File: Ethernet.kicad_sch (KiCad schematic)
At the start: 23 parts, among them T1 WE-RJ45_7499010211A, U4 DP83825IRMQR, Y3 ECS-250-12-33-AGN-TR

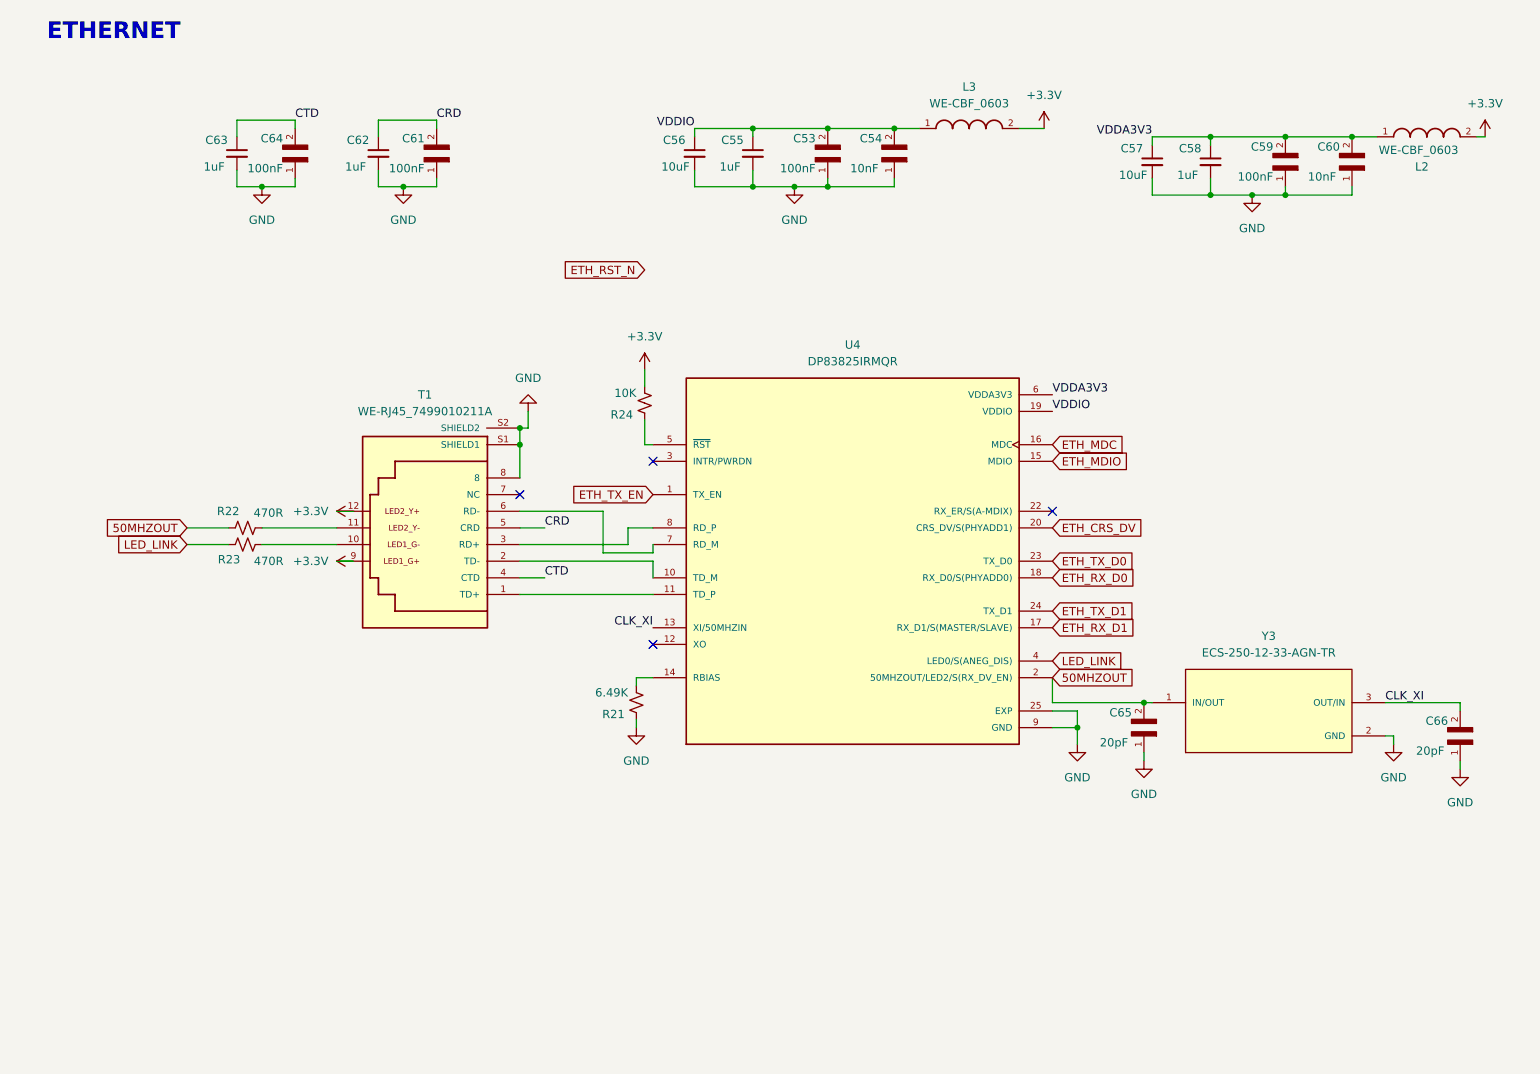
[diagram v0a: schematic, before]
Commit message: schamtic Update
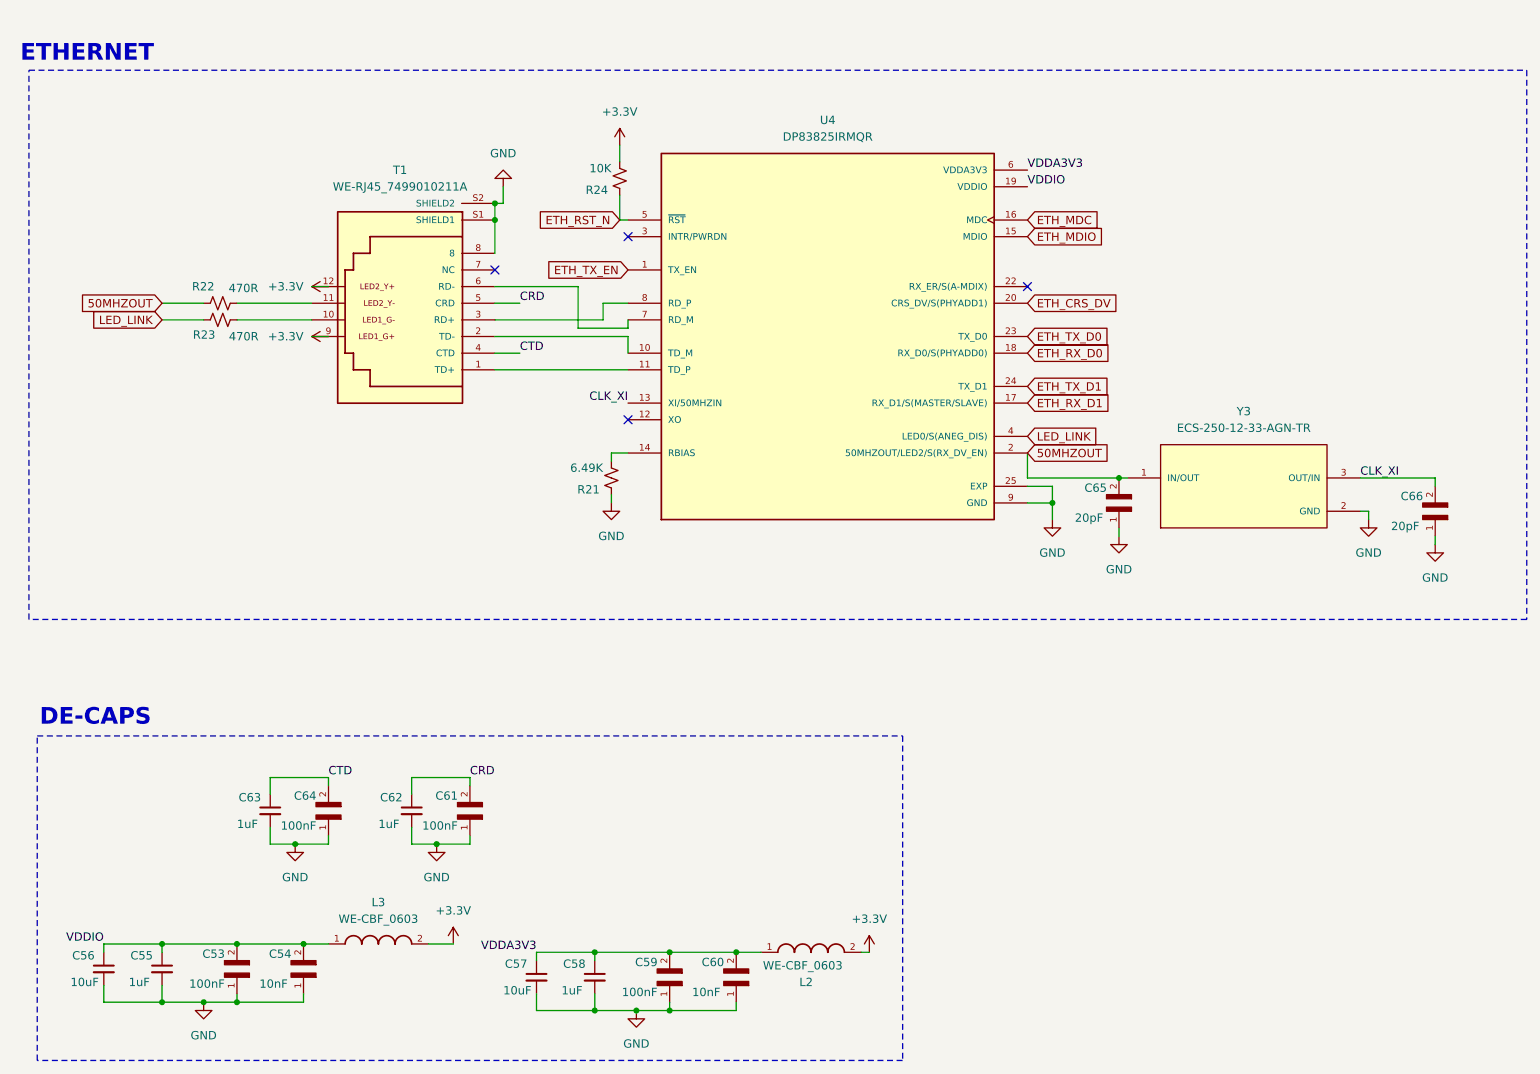
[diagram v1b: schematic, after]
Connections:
- net ETH_RST_N: now also R24.1, U4.5 (~{RST})
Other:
- note added: "DE-CAPS"
- moved on the sheet: C53, C54, C55, C56, C57, C58, C59, C60, C61, C62, C63, C64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
